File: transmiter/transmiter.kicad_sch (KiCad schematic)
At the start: 56 parts, among them J1 USB_B_Mini, J2 Conn_01x04_Pin, J3 Conn_01x04_Pin, SW1 SW_Push, SW2 SW_SPDT, U2 STM32F303K8Tx, U3 AMS1117-3.3, Y1 16MHz

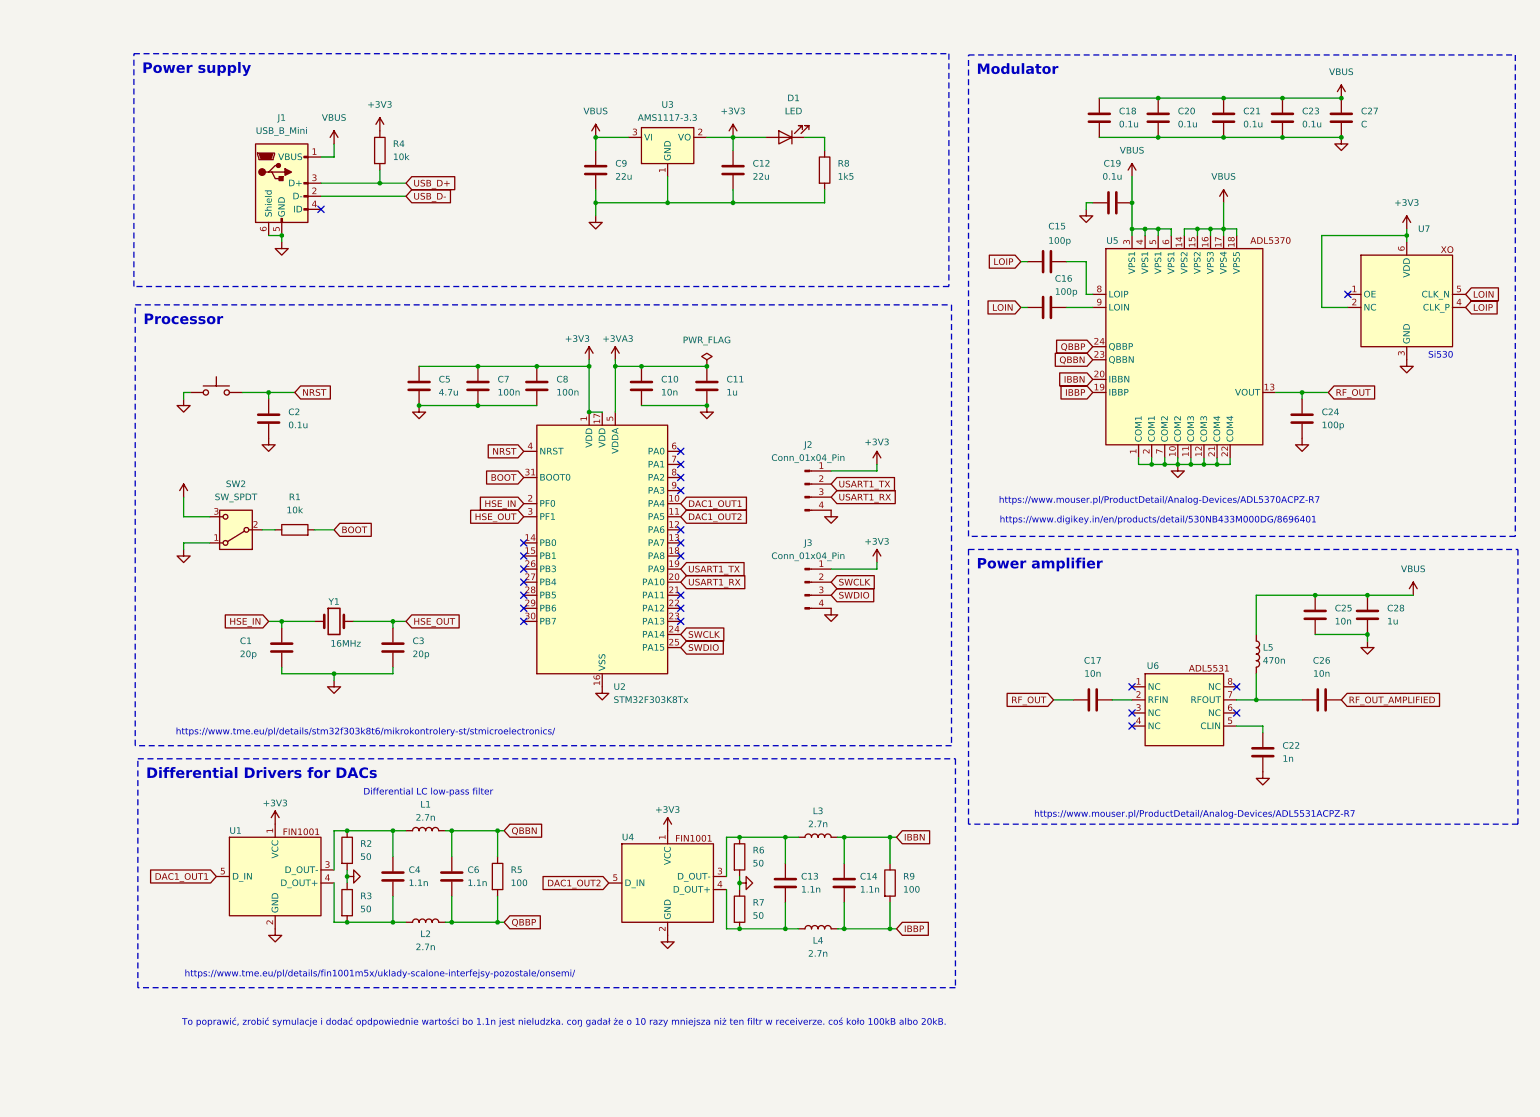
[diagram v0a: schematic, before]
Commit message: First stage of PCB design
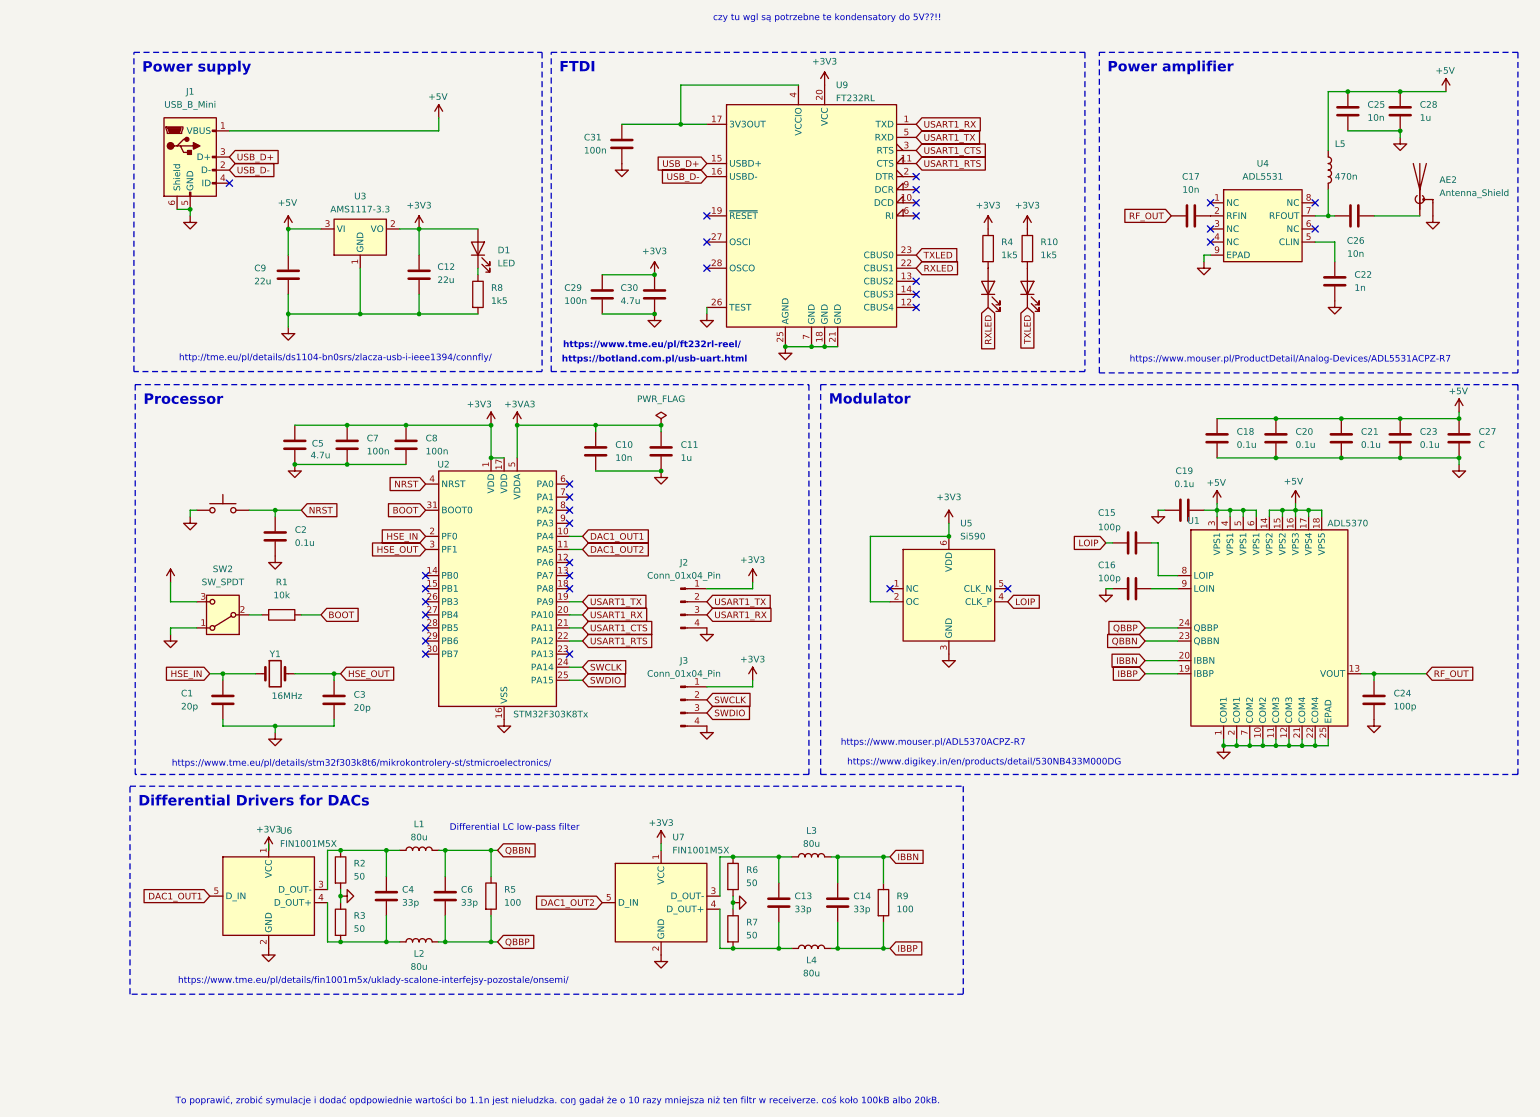
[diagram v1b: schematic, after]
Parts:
- removed U1, U4: ~, Package_TO_SOT_SMD:SOT-23-5_HandSoldering, symbol communication_circuit:FIN1001M5X
- removed U5: ~, Package_CSP:LFCSP-24-1EP_4x4mm_P0.5mm_EP2.3x2.3mm, symbol communication_circuit:ADL5370
- removed U6: ~, symbol communication_circuit:ADL5531
- removed U7: ~, symbol communication_circuit:crystal
- added AE2: Antenna_Shield, Connector_Coaxial:U.FL_Hirose_U.FL-R-SMT-1_Vertical, symbol Device:Antenna_Shield
- added C29, C31: 100n, Capacitor_SMD:C_0603_1608Metric_Pad1.08x0.95mm_HandSolder, symbol Device:C
- added C30: 4.7u, Capacitor_SMD:C_0603_1608Metric_Pad1.08x0.95mm_HandSolder, symbol Device:C
- added D2, D3: LED, LED_SMD:LED_0805_2012Metric_Pad1.15x1.40mm_HandSolder, symbol Device:LED
- added R10: 1k5, Resistor_SMD:R_0603_1608Metric_Pad0.98x0.95mm_HandSolder, symbol Device:R
- added U1: ADL5370, Package_CSP:LFCSP-24-1EP_4x4mm_P0.5mm_EP2.3x2.3mm, symbol Communication_circuit:ADL5370
- added U4: ADL5531, Package_CSP:LFCSP-8-1EP_3x3mm_P0.5mm_EP1.45x1.74mm, symbol Communication_circuit:ADL5531
- added U5: Si590, Oscillator:Oscillator_SMD_IDT_JU6-6_7.0x5.0mm_P2.54mm, symbol Communication_circuit:Si590
- added U6, U7: FIN1001M5X, Package_TO_SOT_SMD:SOT-23-5_HandSoldering, symbol Communication_circuit:FIN1001M5X
- added U9: FT232RL, Package_SO:SSOP-28_5.3x10.2mm_P0.65mm, symbol Interface_USB:FT232RL
- C13, C14, C4, C6: value 1.1n -> 33p
- C15, C16, C17, C18, C19, C20, C21, C23, C24, C27: footprint Capacitor_SMD:C_0603_1608Metric_Pad1.08x0.95mm_HandSolder -> Capacitor_SMD:C_0402_1005Metric_Pad0.74x0.62mm_HandSolder
- J1: footprint Connector_USB:USB_B_Lumberg_2411_02_Horizontal -> Connector_USB:USB_Mini-B_Lumberg_2486_01_Horizontal
- L1, L2, L3, L4: value 2.7n -> 80u
- L5: footprint Inductor_SMD:L_0603_1608Metric_Pad1.05x0.95mm_HandSolder -> Inductor_SMD:L_1008_2520Metric_Pad1.43x2.20mm_HandSolder
- R4: value 10k -> 1k5
- SW1: footprint (none) -> Communication_circuit:PUSH
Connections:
- net LOIN is gone; now on net GND: C16.2
- net +3V3: now also C29.2, C30.2, R10.1, U5.2 (OC), U5.6 (VDD), U6.1 (VCC), U7.1 (VCC), U9.20 (VCC)
- net DAC1_OUT1: now also U6.5 (D_IN)
- net DAC1_OUT2: now also U7.5 (D_IN)
- net GND: now also C9.1, AE2.2 (Shield), C29.1, C30.1, C31.1, U1.1 (COM1), U1.10 (COM2), U1.11 (COM3), U1.12 (COM3), U1.2 (COM1), U1.21 (COM4), U1.22 (COM4), U1.25 (EPAD), U1.7 (COM2), U4.9 (EPAD), U5.3 (GND), U6.2 (GND), U7.2 (GND), U9.18 (GND), U9.21 (GND), U9.25 (AGND), U9.26 (TEST), U9.7 (GND); no longer C9.2
- net IBBN: now also U1.20 (IBBN)
- net IBBP: now also U1.19 (IBBP)
- net LOIP: now also U5.4 (CLK_P)
- net QBBN: now also U1.23 (QBBN)
- net QBBP: now also U1.24 (QBBP)
- net RF_OUT: now also U1.13 (VOUT)
- net USART1_RX: now also U9.1 (TXD)
- net USART1_TX: now also U9.5 (RXD)
- net USB_D+: now also U9.15 (USBD+); no longer R4.2
- net USB_D-: now also U9.16 (USBD-)
- net at C13.1, L3.1, R6.1: now also U7.3 (D_OUT-)
- net at C13.2, L4.1, R7.2: now also U7.4 (D_OUT+)
- net at C4.2, L2.1, R3.2: now also U6.4 (D_OUT+)
- net at C26.1, L5.2: now also U4.7 (RFOUT)
- net at C16.1: now also U1.9 (LOIN)
- net at C4.1, L1.1, R2.1: now also U6.3 (D_OUT-)
- net USART1_CTS: now reaches U2.21 (PA11)
- net USART1_CTS: now also U9.3 (RTS)
- net USART1_RTS: now reaches U2.22 (PA12)
- net USART1_RTS: now also U9.11 (CTS)
- net at C15.1: now also U1.8 (LOIP)
- net at C17.2: now also U4.2 (RFIN)
- net at C22.1: now also U4.5 (CLIN)
- net RF_OUT_AMPLIFIED: no longer names the net of C26.2
- net RF_OUT_AMPLIFIED: now also AE2.1 (A)
- net VBUS renamed +5V
- net +5V: now also C9.2, U1.14 (VPS2), U1.15 (VPS2), U1.16 (VPS3), U1.17 (VPS4), U1.18 (VPS5), U1.3 (VPS1), U1.4 (VPS1), U1.5 (VPS1), U1.6 (VPS1); no longer C9.1
- new net: D3.2 (A), R10.2
- new net: D2.2 (A), R4.2
- new net: C31.2, U9.17 (3V3OUT), U9.4 (VCCIO)
- new net RXLED: D2.1 (K), U9.22 (CBUS1)
- new net TXLED: D3.1 (K), U9.23 (CBUS0)
- no-connect marks 24 -> 33
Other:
- note added: "czy tu wgl są potrzebne te kondensatory do 5V??!!"
- note added: "http://tme.eu/pl/details/ds1104-bn0srs/zlacza-usb-i-ieee1394/connfly/"
- note added: "https://botland.com.pl/usb-uart.html"
- note added: "https://www.digikey.in/en/products/detail/530NB433M000DG"
- note added: "https://www.mouser.pl/ADL5370ACPZ-R7"
- note added: "https://www.tme.eu/pl/ft232rl-reel/"
- note removed: "Si530"
- note removed: "https://www.digikey.in/en/products/detail/530NB433M000DG/8696401"
- note removed: "https://www.mouser.pl/ProductDetail/Analog-Devices/ADL5370ACPZ-R7"
- moved on the sheet: C1, C10, C11, C12, C13, C14, C15, C16, C17, C18, C19, C2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

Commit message: Finished PCB design
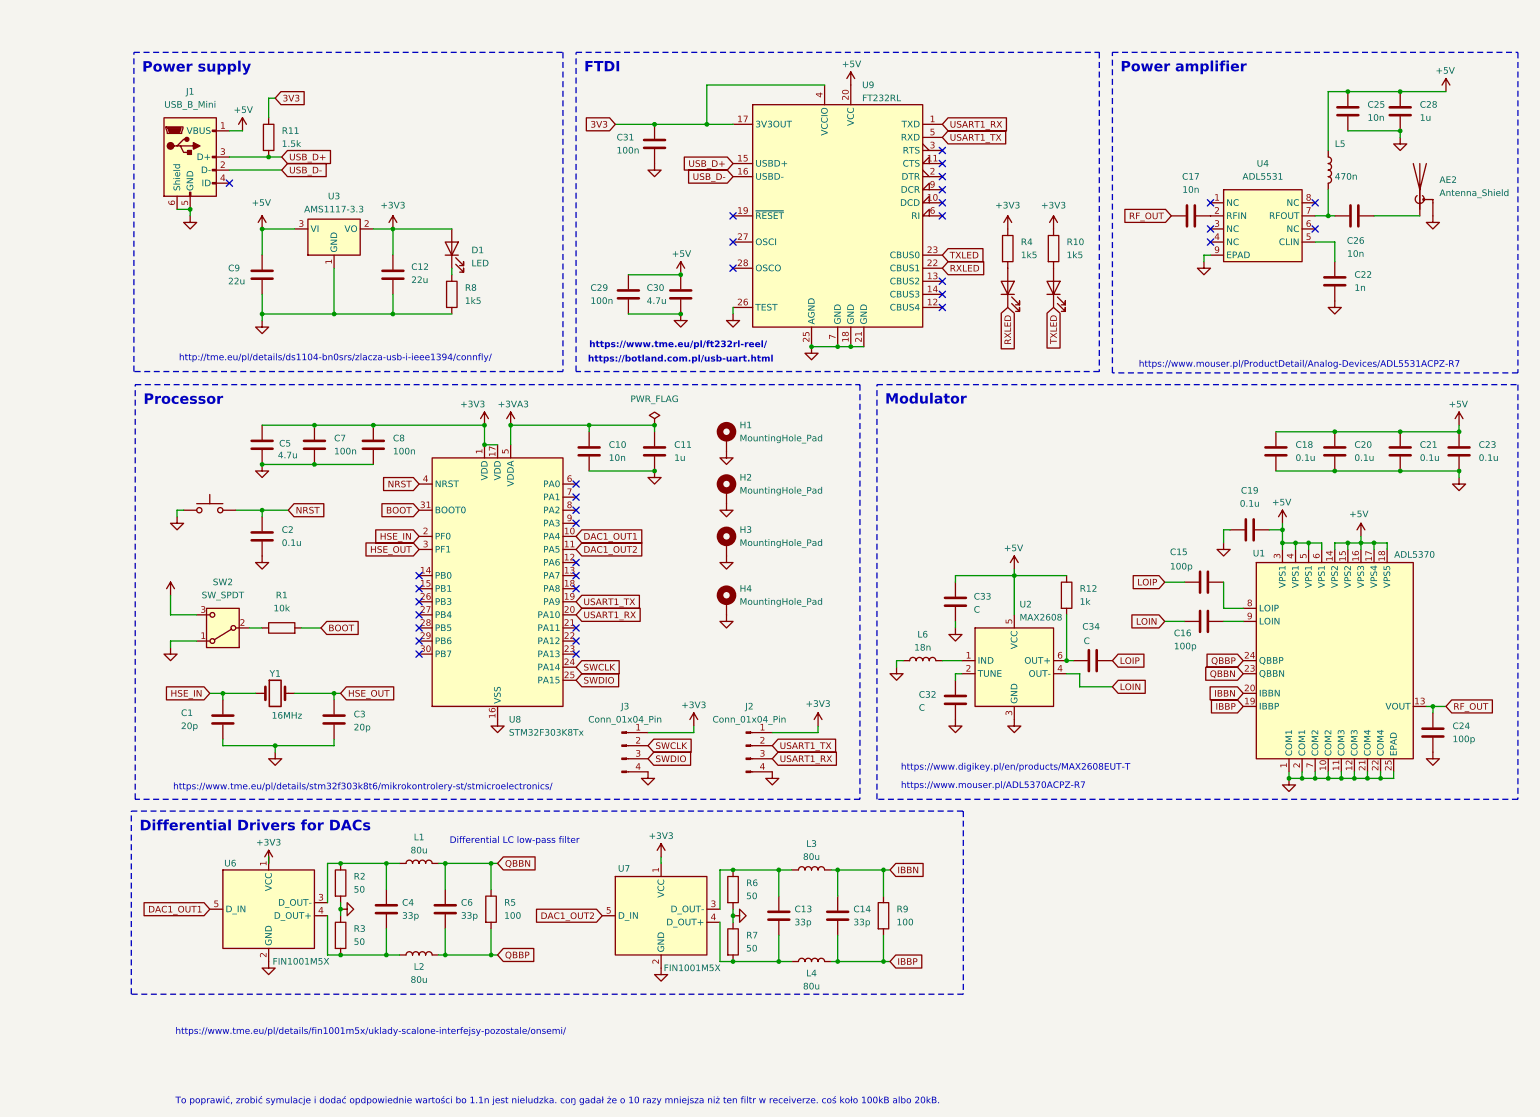
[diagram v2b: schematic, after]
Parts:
- removed C27: C, Capacitor_SMD:C_0402_1005Metric_Pad0.74x0.62mm_HandSolder, symbol Device:C
- removed U2: STM32F303K8Tx, Package_QFP:LQFP-32_7x7mm_P0.8mm, symbol MCU_ST_STM32F3:STM32F303K8Tx
- removed U5: Si590, Oscillator:Oscillator_SMD_IDT_JU6-6_7.0x5.0mm_P2.54mm, symbol Communication_circuit:Si590
- added C32, C33, C34: C, Capacitor_SMD:C_0603_1608Metric_Pad1.08x0.95mm_HandSolder, symbol Device:C
- added H1, H2, H3, H4: MountingHole_Pad, MountingHole:MountingHole_2.2mm_M2_DIN965_Pad, symbol Mechanical:MountingHole_Pad
- added L6: 18n, Inductor_SMD:L_0603_1608Metric_Pad1.05x0.95mm_HandSolder, symbol Device:L
- added R11: 1.5k, Resistor_SMD:R_0603_1608Metric_Pad0.98x0.95mm_HandSolder, symbol Device:R
- added R12: 1k, Resistor_SMD:R_0603_1608Metric_Pad0.98x0.95mm_HandSolder, symbol Device:R
- added U2: MAX2608, Package_TO_SOT_SMD:SOT-23-6, symbol Communication_circuit:MAX2608
- added U8: STM32F303K8Tx, Package_QFP:LQFP-32_7x7mm_P0.8mm, symbol MCU_ST_STM32F3:STM32F303K8Tx
- AE2: footprint Connector_Coaxial:U.FL_Hirose_U.FL-R-SMT-1_Vertical -> Connector_Coaxial:U.FL_Molex_MCRF_73412-0110_Vertical
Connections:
- net +3V3: now also U8.1 (VDD), U8.17 (VDD); no longer C29.2, C30.2, U9.20 (VCC)
- net +3VA3: now also U8.5 (VDDA)
- net +5V: now also C29.2, C30.2, U9.20 (VCC), C33.2, R12.1, U2.5 (VCC)
- net BOOT: now also U8.31 (BOOT0)
- net DAC1_OUT1: now also U8.10 (PA4)
- net DAC1_OUT2: now also U8.11 (PA5)
- net GND: now also C32.1, C33.1, H1.1, H2.1, H3.1, H4.1, L6.1, U2.3 (GND), U8.16 (VSS), U8.32 (VSS); no longer C16.2
- net HSE_IN: now also U8.2 (PF0)
- net HSE_OUT: now also U8.3 (PF1)
- net LOIP: now also C34.2
- net NRST: now also U8.4 (NRST)
- net SWCLK: now also U8.24 (PA14)
- net SWDIO: now also U8.25 (PA15)
- net USART1_RX: now also U8.20 (PA10)
- net USART1_TX: now also U8.19 (PA9)
- net USB_D+: now also R11.2
- net 3V3: now reaches C31.2, U9.17 (3V3OUT), U9.4 (VCCIO)
- net 3V3: now also R11.1
- net USART1_CTS: no longer names the net of U9.3 (RTS)
- net USART1_RTS: no longer names the net of U9.11 (CTS)
- new net: C32.2, U2.2 (TUNE)
- new net: C34.1, R12.2, U2.6 (OUT+)
- new net: L6.2, U2.1 (IND)
- new net LOIN: C16.2, U2.4 (OUT-)
- no-connect marks 33 -> 35
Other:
- note added: "https://www.digikey.pl/en/products/MAX2608EUT-T"
- note removed: "czy tu wgl są potrzebne te kondensatory do 5V??!!"
- note removed: "https://www.digikey.in/en/products/detail/530NB433M000DG"
- moved on the sheet: C1, C10, C11, C12, C13, C14, C15, C16, C18, C19, C2, C20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
